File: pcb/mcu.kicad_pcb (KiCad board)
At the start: 2 copper layers, 35 x 70.5 mm, 10 parts, among them J1 N!N, J2 Conn_01x12_Socket, J3 Conn_01x12_Socket, J6 Display_nice-view, SW37 SW_Push, SW38 RotaryEncoder_Switch, U1 RollerEncoder_EVQWGD001

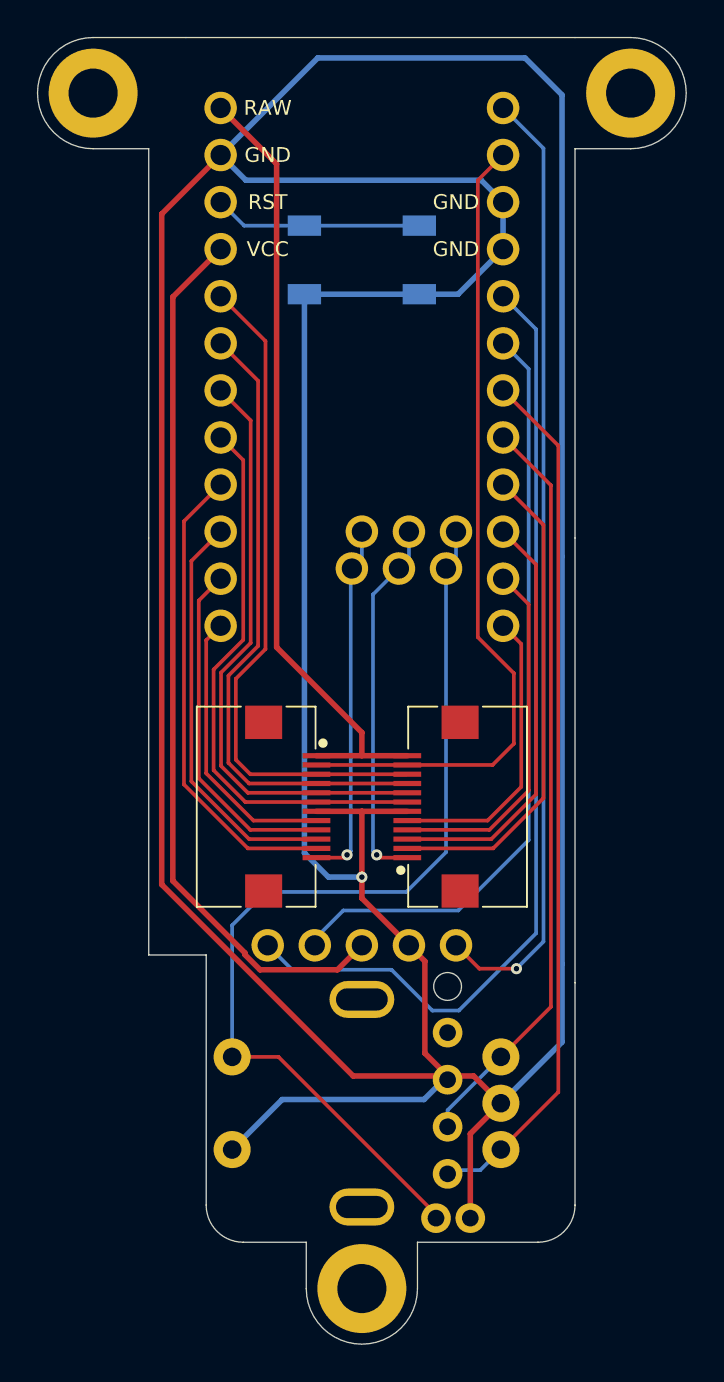
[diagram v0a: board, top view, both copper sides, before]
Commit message: update case and main pcb
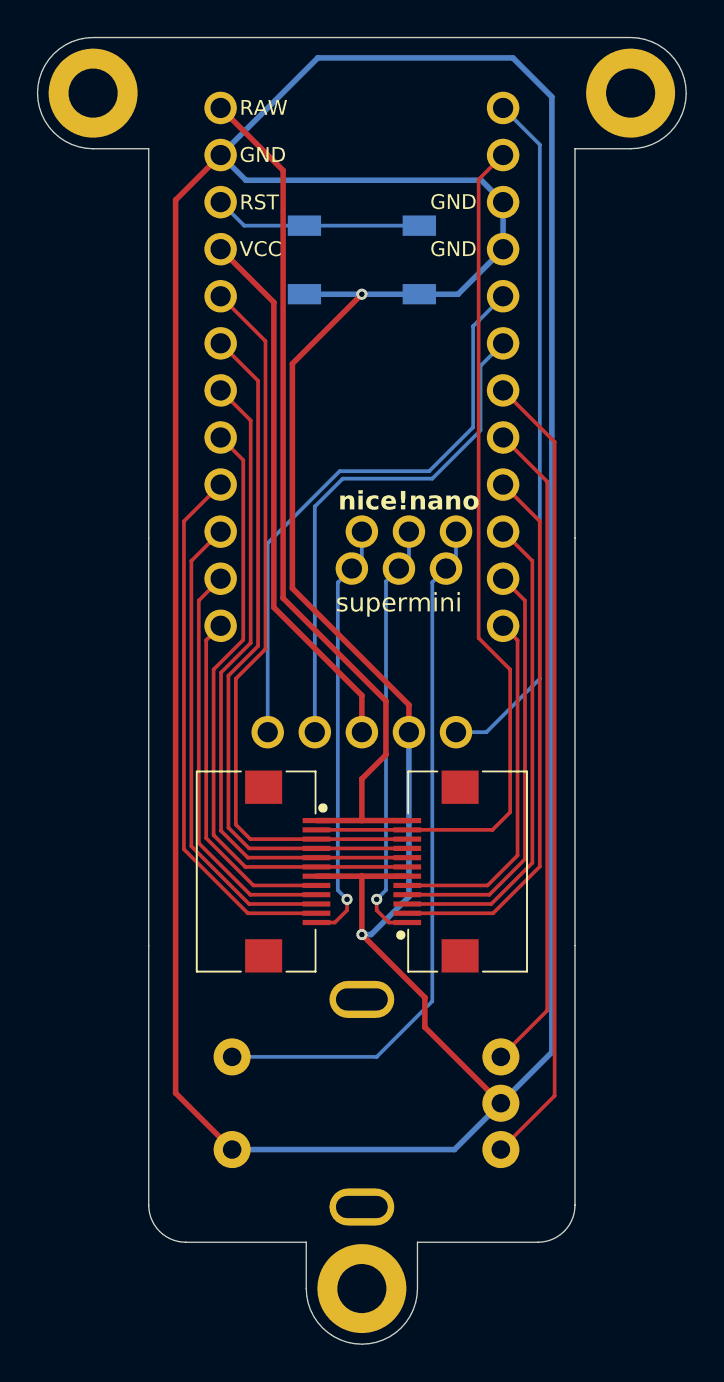
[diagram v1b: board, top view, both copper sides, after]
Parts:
- removed U1: RollerEncoder_EVQWGD001, zzkeeb:RotaryEncoder_EVQWGD001
- moved J6 11.5 mm to (74.0, 60.5)
- moved J2 3.50 mm to (70.0, 84.5)
- moved J3 3.50 mm to (78.0, 84.5)
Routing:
- net (no net): track 426.2 -> 482.1 mm
- net MOSI: track 52.8 -> 31.6 mm
- net +3.3V: track 47.9 -> 29.2 mm
- net OFF: track 52.3 -> 37.9 mm
- net CS: track 51.7 -> 37.3 mm, vias 1 -> 0
- net SCK: track 41.5 -> 28.0 mm
- net GND: track 246.4 -> 238.7 mm, vias 1 -> 2
- net encB: track 40.4 -> 35.4 mm
- net encA: track 46.8 -> 43.3 mm
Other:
- outline, holes or cut-outs redrawn
- board text added: "molekula"
- board text added: "v0.2"
